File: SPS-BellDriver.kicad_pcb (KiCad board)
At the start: 2 copper layers, 54 x 104 mm, 61 parts, among them IC1 TSR_1-2433, J1 Jack-DC, J2 Screw_Terminal_01x02, J3 Screw_Terminal_01x02, J4 Screw_Terminal_01x02, J5 Screw_Terminal_01x05, J6 Screw_Terminal_01x02, J7 Screw_Terminal_01x02, J8 Screw_Terminal_01x05, J9 Screw_Terminal_01x02, Q1 TIP120, Q2 TIP120, Q3 TIP120, Q4 TIP120, Q5 TIP120, Q6 TIP120

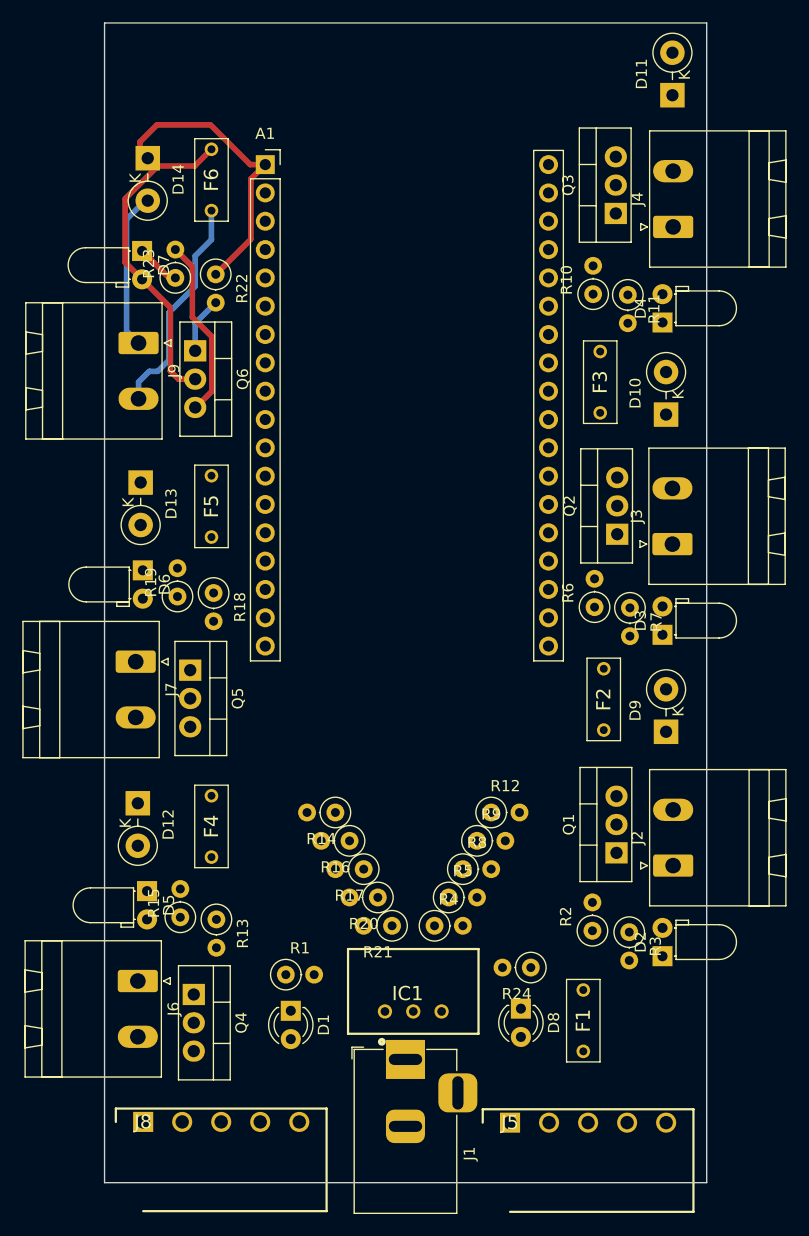
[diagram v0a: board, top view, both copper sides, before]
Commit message: updates
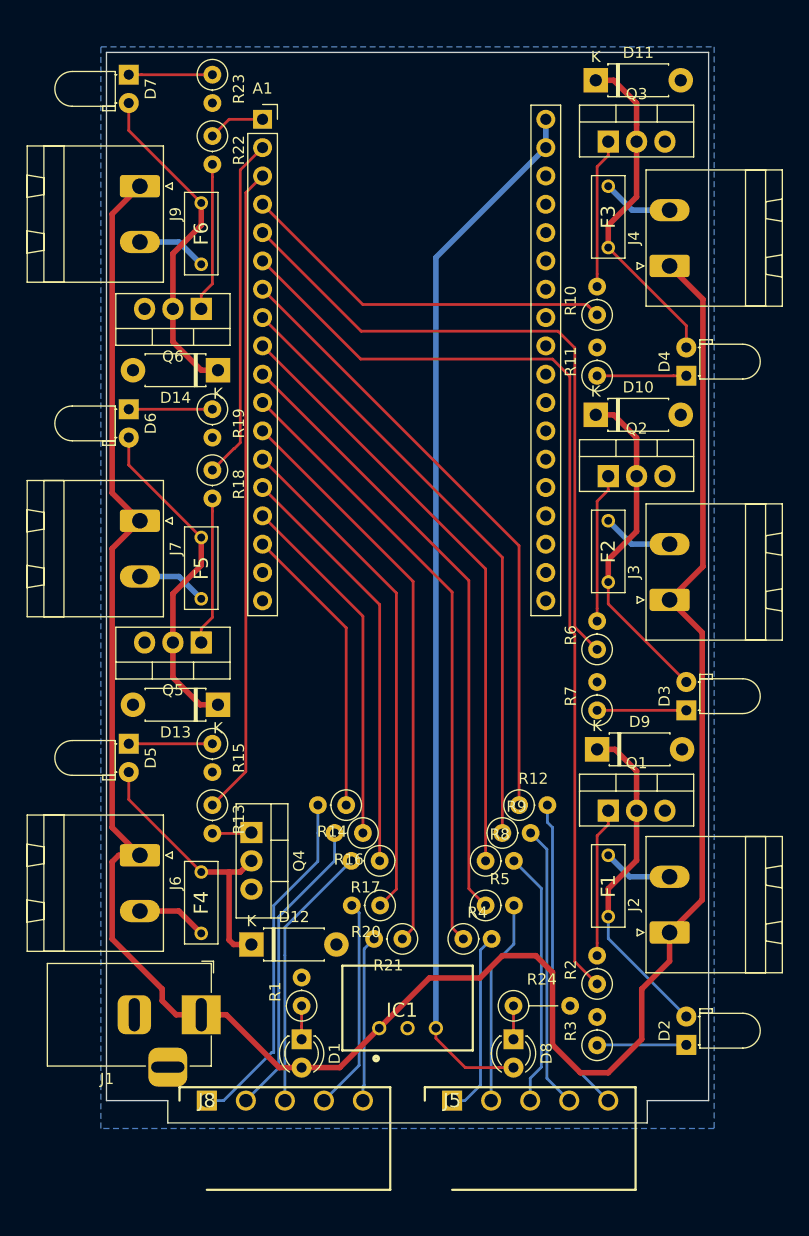
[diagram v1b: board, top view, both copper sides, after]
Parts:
- added H1: 1590B, SamacSys_Parts:1590B, F.Cu at (28.0, 19.0)
- D10, D11, D12, D13, D14, D9: footprint Diode_THT:D_DO-41_SOD81_P3.81mm_Vertical_KathodeUp -> Diode_THT:D_DO-41_SOD81_P7.62mm_Horizontal
- R24: footprint Resistor_THT:R_Axial_DIN0207_L6.3mm_D2.5mm_P2.54mm_Vertical -> Resistor_THT:R_Axial_DIN0207_L6.3mm_D2.5mm_P5.08mm_Vertical
- moved D13 21.1 mm to (39.0, 84.0), turned to 180 degrees
- moved D14 20.0 mm to (39.0, 54.0), turned to 180 degrees
- moved J1 18.7 mm to (37.5, 111.8), turned to 0 degrees
- moved R23 18.5 mm to (38.5, 27.5), turned to 270 degrees
- moved F1 17.7 mm to (74.0, 97.5), turned to 270 degrees
- moved R19 17.1 mm to (38.5, 57.5), turned to 270 degrees
- moved D12 16.3 mm to (42.0, 105.5), turned to 0 degrees
- moved D7 15.9 mm to (31.0, 27.5)
- moved R15 15.8 mm to (38.5, 87.5), turned to 270 degrees
- moved Q4 15.4 mm to (42.0, 95.5)
- moved F3 14.8 mm to (74.0, 37.5)
- moved D6 14.5 mm to (31.0, 57.5)
- moved J9 14.1 mm to (32.0, 37.5)
- moved D5 13.3 mm to (31.0, 87.5)
- moved F2 13.3 mm to (74.0, 67.5)
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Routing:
- net /V_in: track 13.2 -> 215.5 mm
- net /VCC: track 0.00 -> 94.5 mm
- net Net-(A1-Pad6): track 0.00 -> 87.3 mm
- net Net-(A1-Pad5): track 0.00 -> 60.2 mm
- net Net-(A1-Pad3): track 0.00 -> 58.3 mm
- net Net-(A1-Pad10): track 0.00 -> 55.9 mm
- net Net-(A1-Pad7): track 0.00 -> 55.8 mm
- net Net-(A1-Pad11): track 0.00 -> 55.6 mm
- net Net-(A1-Pad8): track 0.00 -> 55.1 mm
- net Net-(A1-Pad9): track 0.00 -> 54.5 mm
- net Net-(A1-Pad12): track 0.00 -> 51.5 mm
- net Net-(A1-Pad13): track 0.00 -> 45.6 mm
- net Net-(A1-Pad14): track 0.00 -> 37.8 mm
- net Net-(A1-Pad4): track 0.00 -> 34.1 mm
- net Net-(A1-Pad15): track 0.00 -> 32.2 mm
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- added copper zone on B.Cu, net GND
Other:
- board size 54 x 104 mm -> 54 x 96 mm
